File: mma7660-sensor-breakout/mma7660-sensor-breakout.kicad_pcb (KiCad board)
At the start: 2 copper layers, 13.5 x 11.7 mm, 4 parts, among them J1 HEADER, U1 MMA7660-DFN10

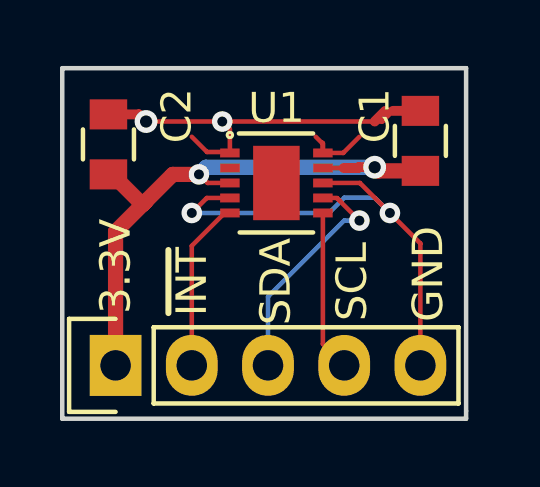
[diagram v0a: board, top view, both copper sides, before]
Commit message: Release v1.1 MMA7660 breakout.
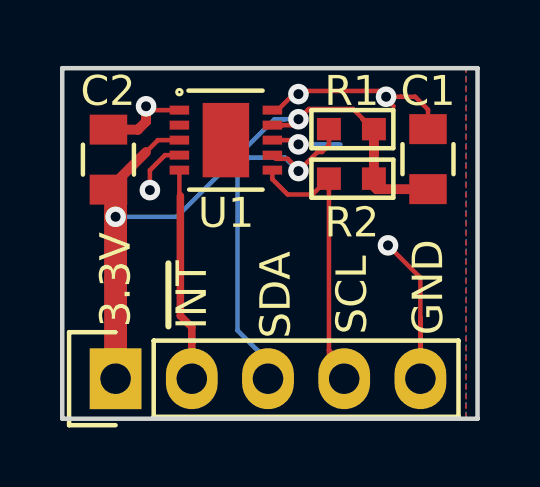
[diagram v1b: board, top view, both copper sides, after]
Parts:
- added R1: 1K, Wickerlib:RLC-0603-SMD, F.Cu at (150.6, 105.4)
- added R2: 1K, Wickerlib:RLC-0603-SMD, F.Cu at (150.6, 107.1)
- U1: value MMA7660-DFN10 -> IC-MMA7660-DFN10
- moved U1 2.21 mm to (146.4, 105.8)
- moved C1 0.66 mm to (153.2, 106.4)
- moved C2 0.51 mm to (142.5, 106.4)
- moved J1 0.44 mm to (142.7, 113.7)
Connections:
- net Net-(J1-Pad2) renamed /INT
- net Net-(J1-Pad3) renamed /SDA
- net Net-(J1-Pad4) renamed /SCL
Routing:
- net GND: track 32.4 -> 21.3 mm, vias 4 -> 6
- net +3V3: track 20.2 -> 28.3 mm
- net /SDA: track 7.91 -> 13.6 mm
- net /SCL: track 5.37 -> 10.2 mm
- net /INT: track 5.71 -> 7.89 mm
- net (no net): track 0.50 -> 0.00 mm
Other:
- board size 13.5 x 11.7 mm -> 13.8 x 11.7 mm
- net class Default: clearance 0.254 -> 0.1524
- rule trace_clearance: 0.254 -> 0.1524
- board text added: "12/31/16"
- board text added: "MMA7660 Breakout Board v1.1"
- board text added: "MMA7660 Breakout v1.1"
- board text removed: "8/30/16"
- board text removed: "MMA7660 Breakout Board v1.0"
- board text removed: "MMA7660 Breakout v1.0"
